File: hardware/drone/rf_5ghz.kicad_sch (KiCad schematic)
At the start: 19 parts, among them J5 Conn_01x06_Pin, U7 CC3350, U8 DPX167125DT-8197B1, U9 DEA162450BT-1295A1, Y1 Crystal_GND24

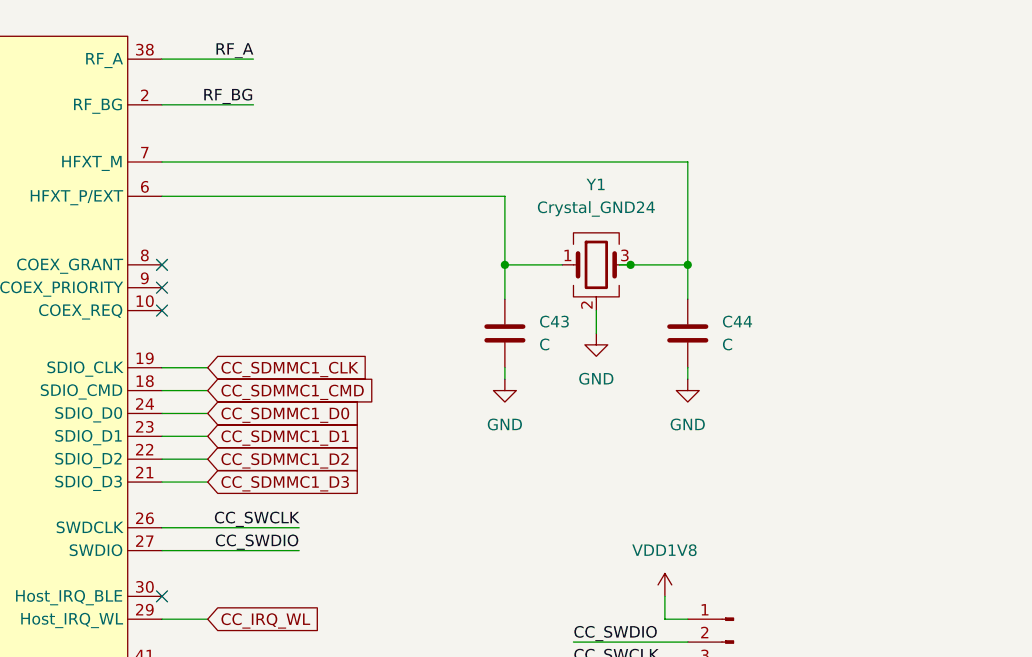
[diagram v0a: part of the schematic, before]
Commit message: Small cleanup
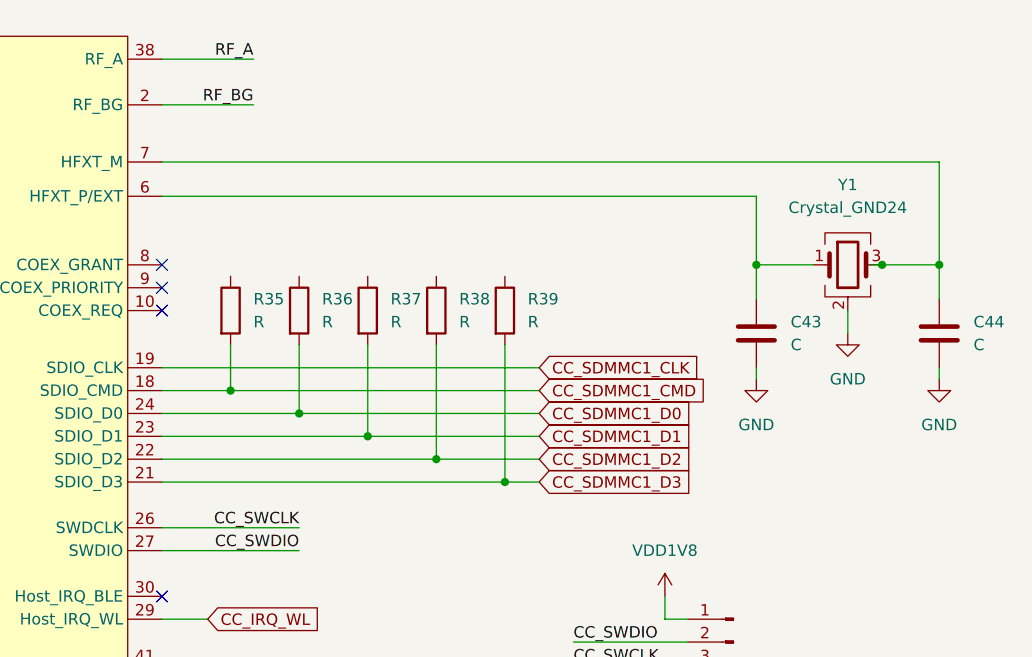
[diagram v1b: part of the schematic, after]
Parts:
- added R35, R36, R37, R38, R39: R, symbol Device:R
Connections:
- net CC_SDMMC1_CMD: now also R35.2
- net CC_SDMMC1_D0: now also R36.2
- net CC_SDMMC1_D1: now also R37.2
- net CC_SDMMC1_D2: now also R38.2
- net CC_SDMMC1_D3: now also R39.2
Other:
- moved on the sheet: C43, C44, Y1
